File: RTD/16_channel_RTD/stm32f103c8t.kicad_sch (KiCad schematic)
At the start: 14 parts, among them SW2 SW_SPDT, U7 STM32F103C8Tx

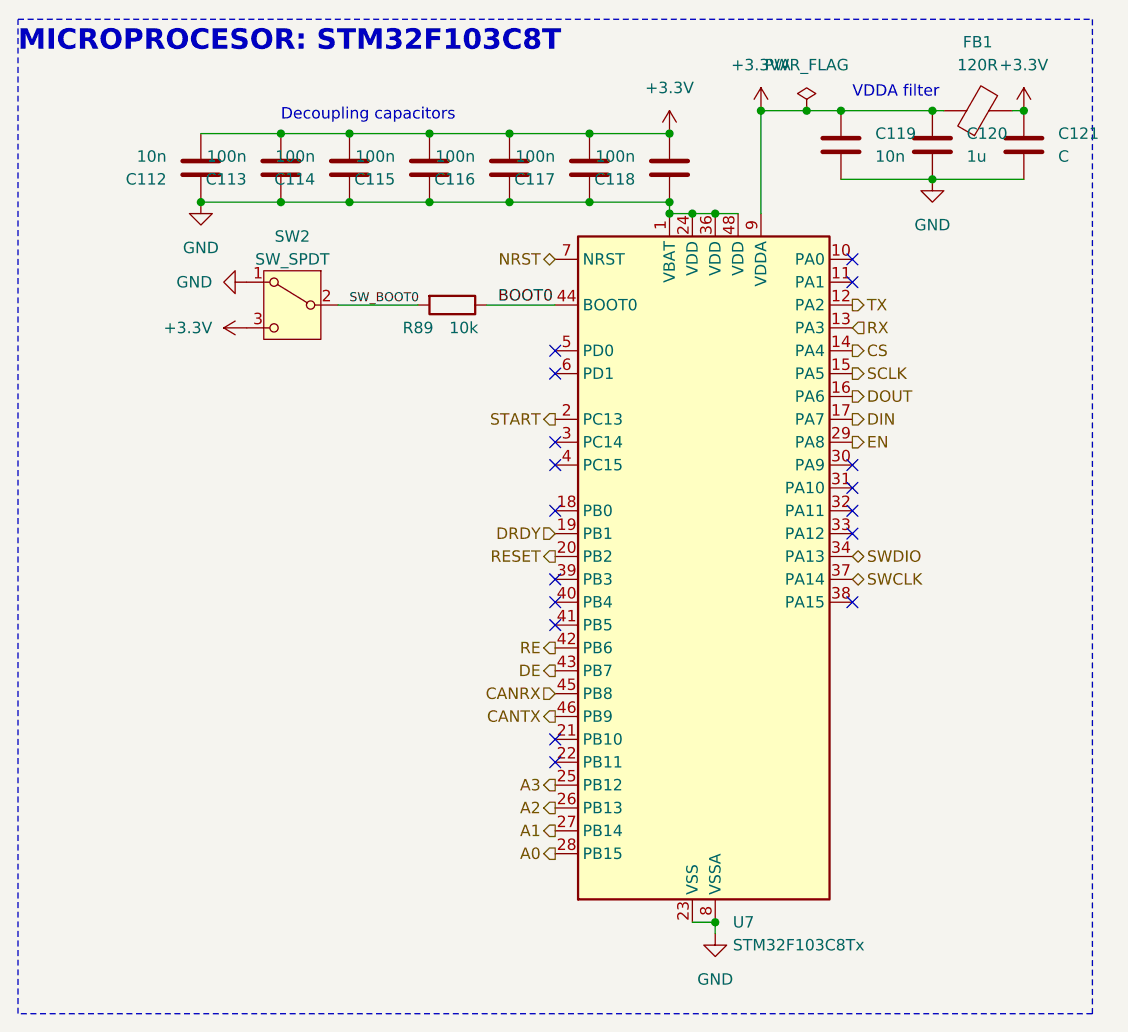
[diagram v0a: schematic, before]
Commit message: ERC free
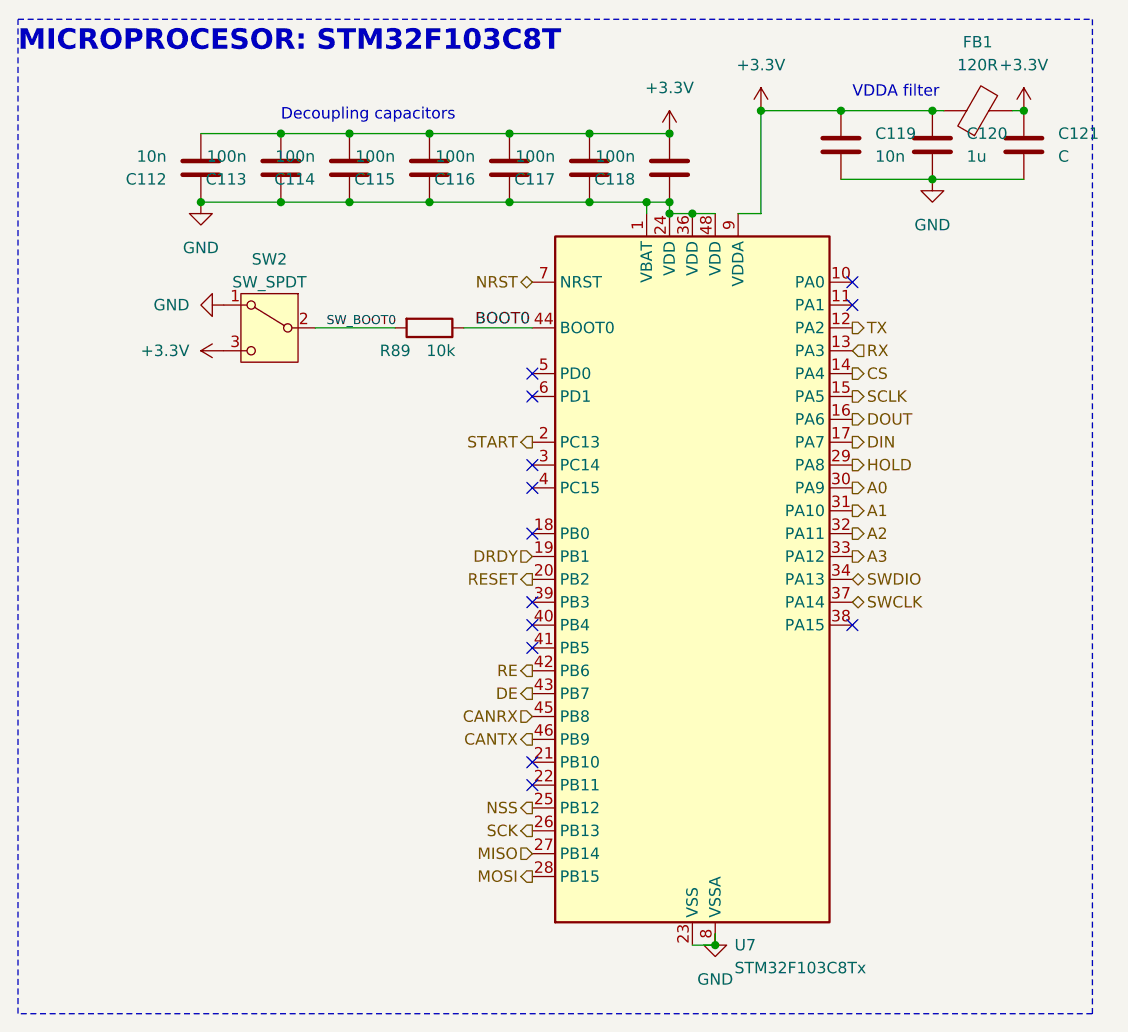
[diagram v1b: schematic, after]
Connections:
- net +3.3VA is gone; now on net +3.3V: C119.1, C120.1, FB1.1, U7.9 (VDDA)
- net A0: now also U7.30 (PA9); no longer U7.28 (PB15)
- net A1: now also U7.31 (PA10); no longer U7.27 (PB14)
- net A2: now also U7.32 (PA11); no longer U7.26 (PB13)
- net A3: now also U7.33 (PA12); no longer U7.25 (PB12)
- net EN renamed HOLD
- new net MISO: U7.27 (PB14)
- new net MOSI: U7.28 (PB15)
- new net NSS: U7.25 (PB12)
- new net SCK: U7.26 (PB13)
- no-connect marks 17 -> 13
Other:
- moved on the sheet: R89, SW2, U7
